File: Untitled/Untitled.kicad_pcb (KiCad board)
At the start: 2 copper layers, 74.3 x 69.9 mm, 80 parts, among them IC1 DRV8210, IC2 TPS7A2033, J1 POWER, J10 PROG, J11 Conn_01x08_Socket, J2 Volume, J3 Input, J4 IR, J5 Motor out, J6 Relays, J7 PGA, J8 Display data, J9 Display Power, U1 ATtiny1616, U11 MCP120, U2 MCP6001, U3 PCA9306, U4 MCP23008

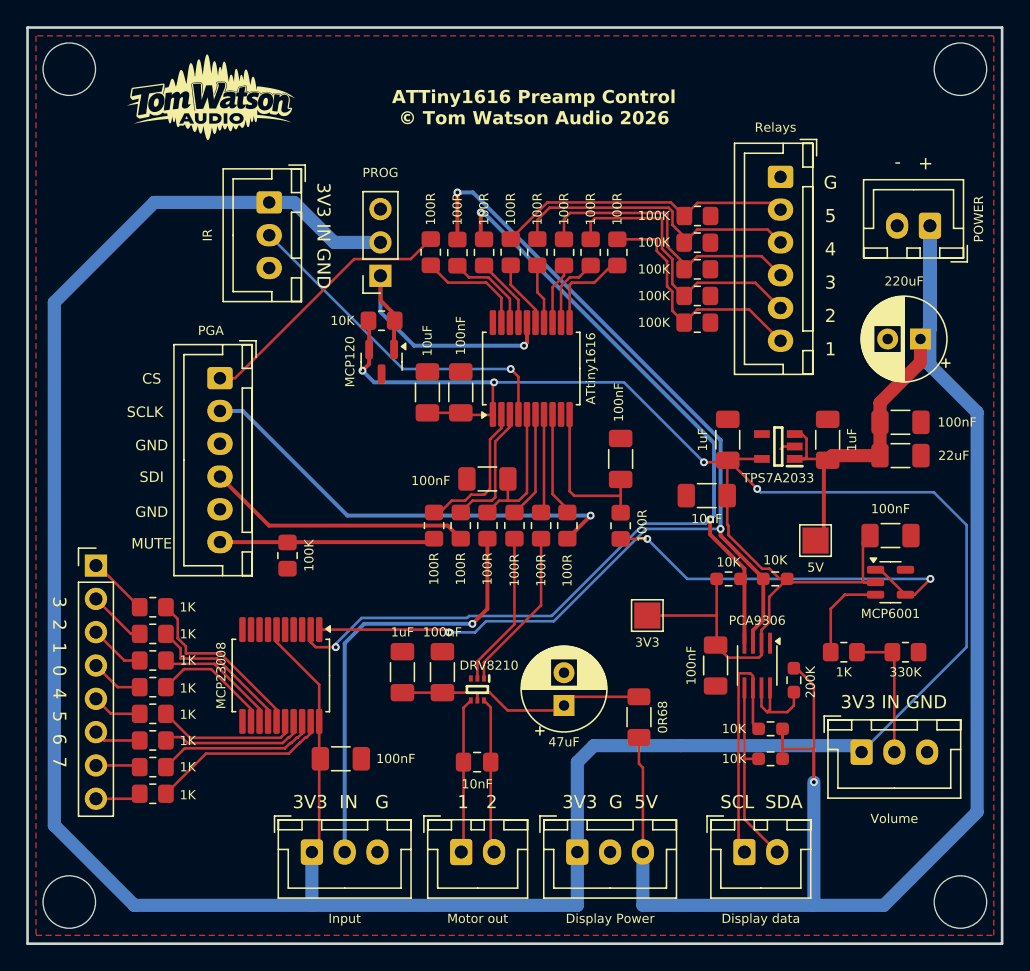
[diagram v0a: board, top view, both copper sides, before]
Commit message: ooo
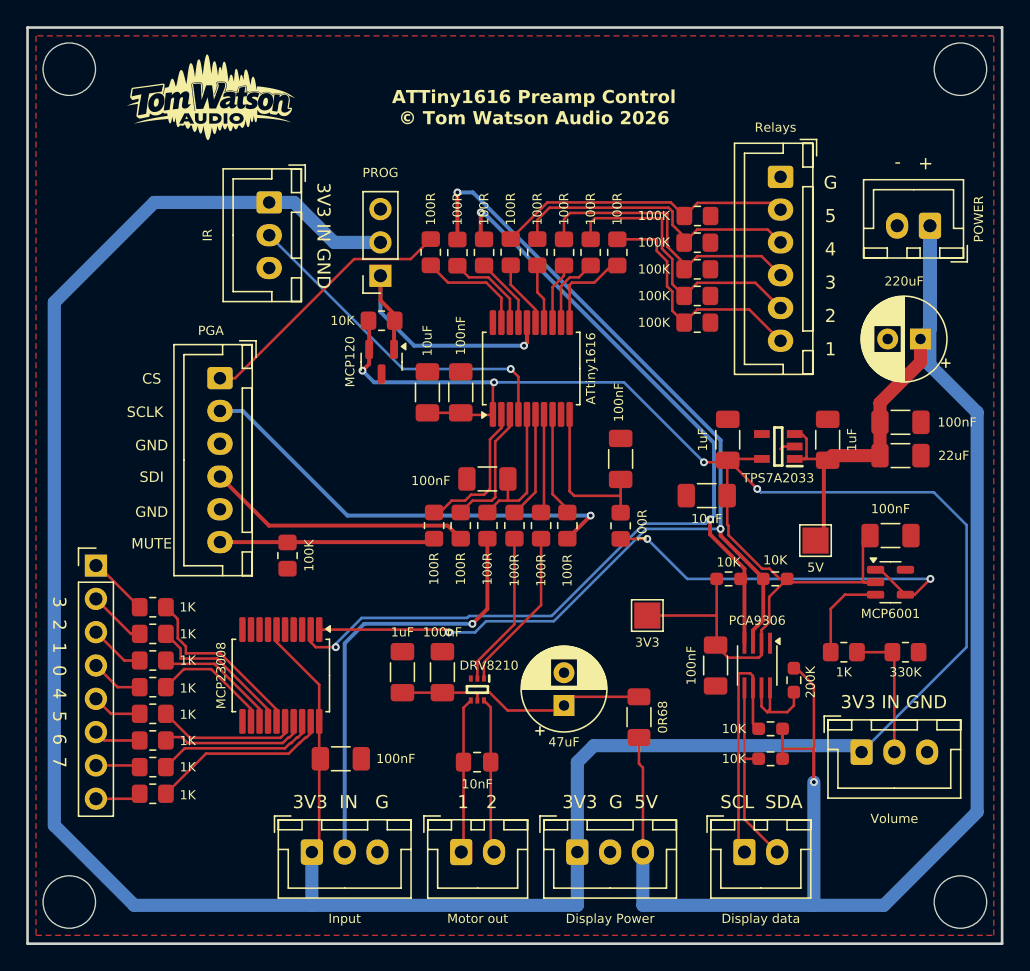
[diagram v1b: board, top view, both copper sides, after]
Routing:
- net /3V3: track 297.5 -> 294.8 mm
- net /5V-IN: track 151.2 -> 149.2 mm
- net /RELAY5: track 23.9 -> 22.1 mm
- net /5V-MOTOR: track 18.8 -> 17.8 mm
- net Net-(U1-PC2): track 5.30 -> 4.58 mm
- net /SCL5V: track 19.2 -> 18.6 mm
- net Net-(J11-Pin_8): track 3.49 -> 2.95 mm
- net /PROG: track 22.7 -> 22.2 mm
